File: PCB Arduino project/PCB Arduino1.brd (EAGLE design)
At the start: 55.9 x 70.8 mm, 7 parts, among them CN1 1X4-BIG

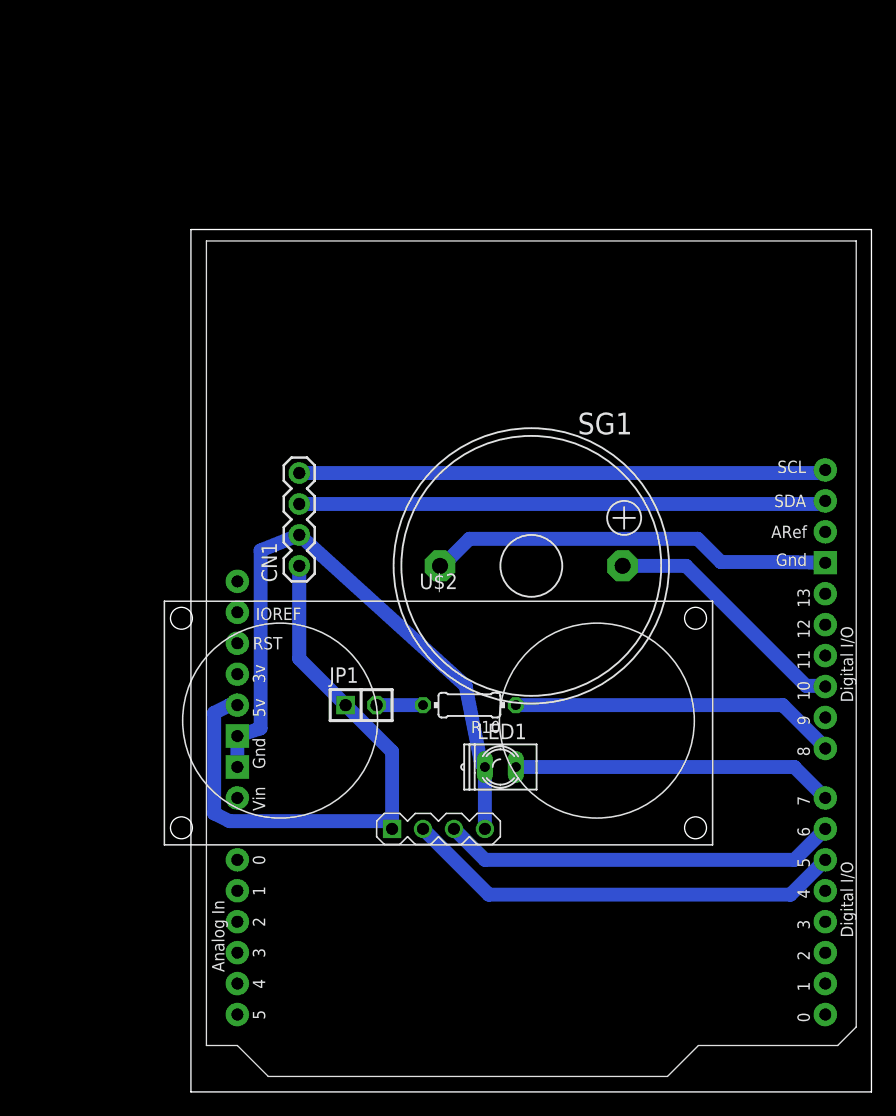
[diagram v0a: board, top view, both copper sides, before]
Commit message: update
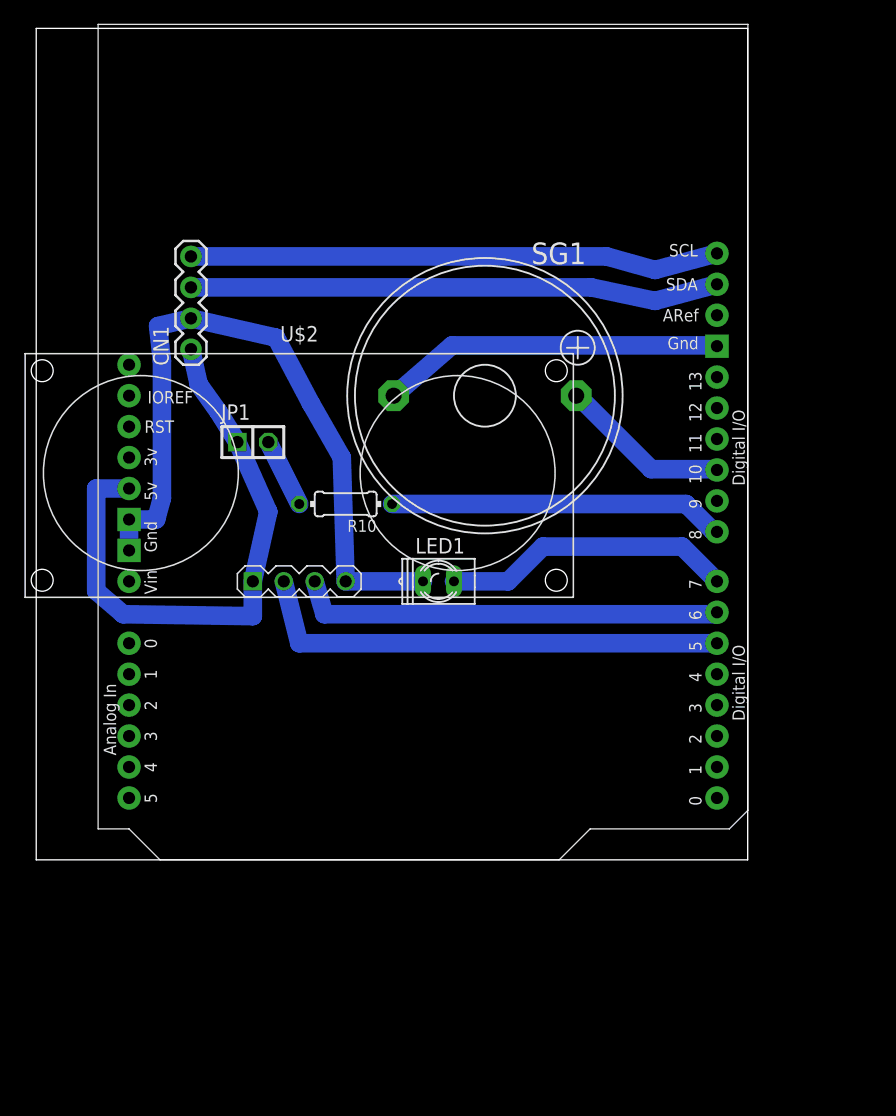
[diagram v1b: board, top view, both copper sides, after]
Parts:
- moved JP1 23.3 mm to (12.7, 66.0)
- moved U$2 23.3 mm to (16.5, 63.5)
- moved U$1 19.9 mm to (26.7, 66.0)
- moved CN1 19.9 mm to (7.62, 73.7)
- moved R10 19.4 mm to (20.3, 61.0)
- moved LED1 16.1 mm to (27.9, 54.6)
- moved SG1 14.5 mm to (31.8, 69.8)
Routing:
- net D10: track 20.8 -> 14.1 mm
- net GND: track 53.0 -> 58.4 mm
- net GND2: track 33.3 -> 28.1 mm
- net D5: track 36.4 -> 39.5 mm
- net D6: track 32.6 -> 35.1 mm
- net D7: track 26.5 -> 24.0 mm
- net 5V: track 50.2 -> 48.3 mm
- net N$1: track 3.81 -> 5.68 mm
- net D8: track 26.9 -> 27.7 mm
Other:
- board size 55.9 x 70.8 mm -> 58.4 x 68.2 mm
